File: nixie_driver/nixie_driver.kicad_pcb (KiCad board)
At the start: 2 copper layers, 39 parts, among them J1 USB_B_Micro, J14 Anode, J15 Number IO, J16 Number IO, J17 Anode, J18 Anode, J19 Number IO, J2 GPIO, J20 Number IO, J21 Anode, J22 Anode, J23 Number IO, J24 Number IO, J25 Anode, J3 HV_TEST, J4 Screw_Terminal_01x02, J5 Number IO, J6 Anode, J7 Number IO, J8 Anode, U1 SN74141N, U2 SN74141N, U3 SN74141N, U4 SN74141N

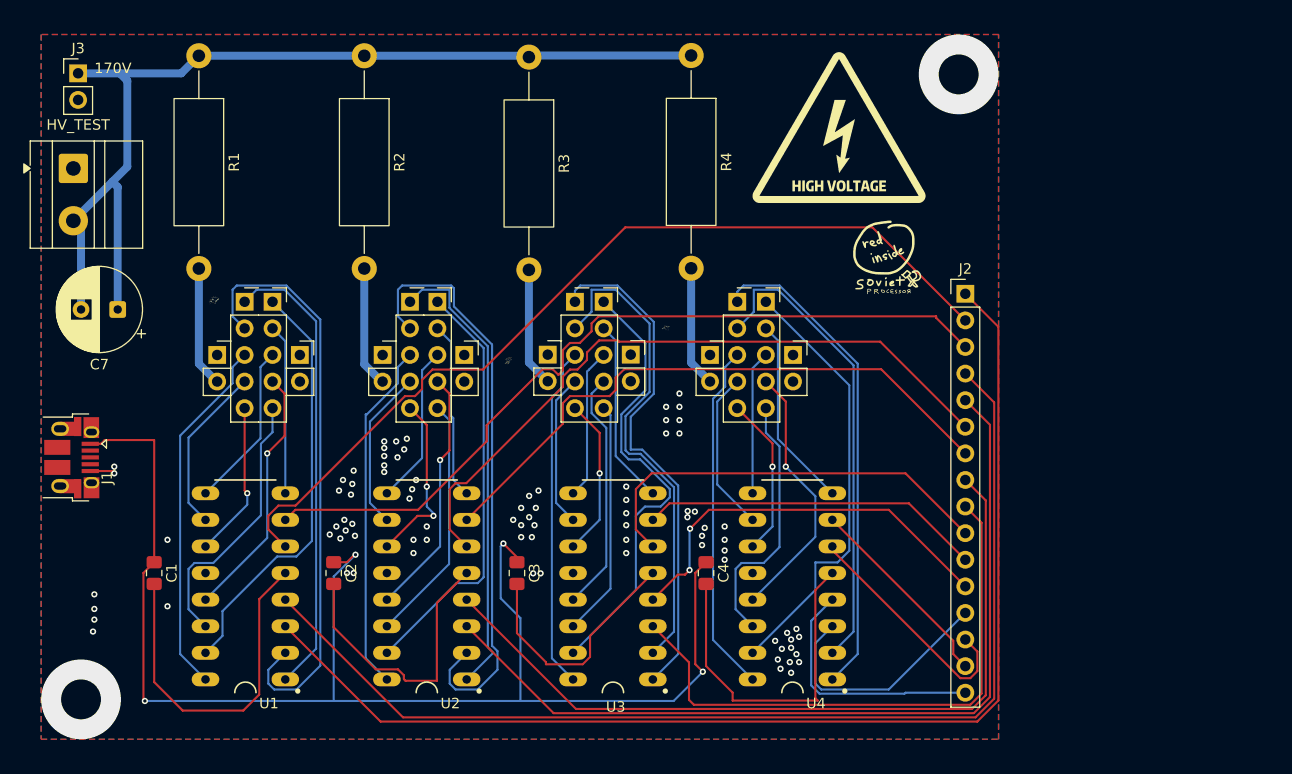
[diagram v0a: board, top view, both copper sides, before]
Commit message: updated pcb
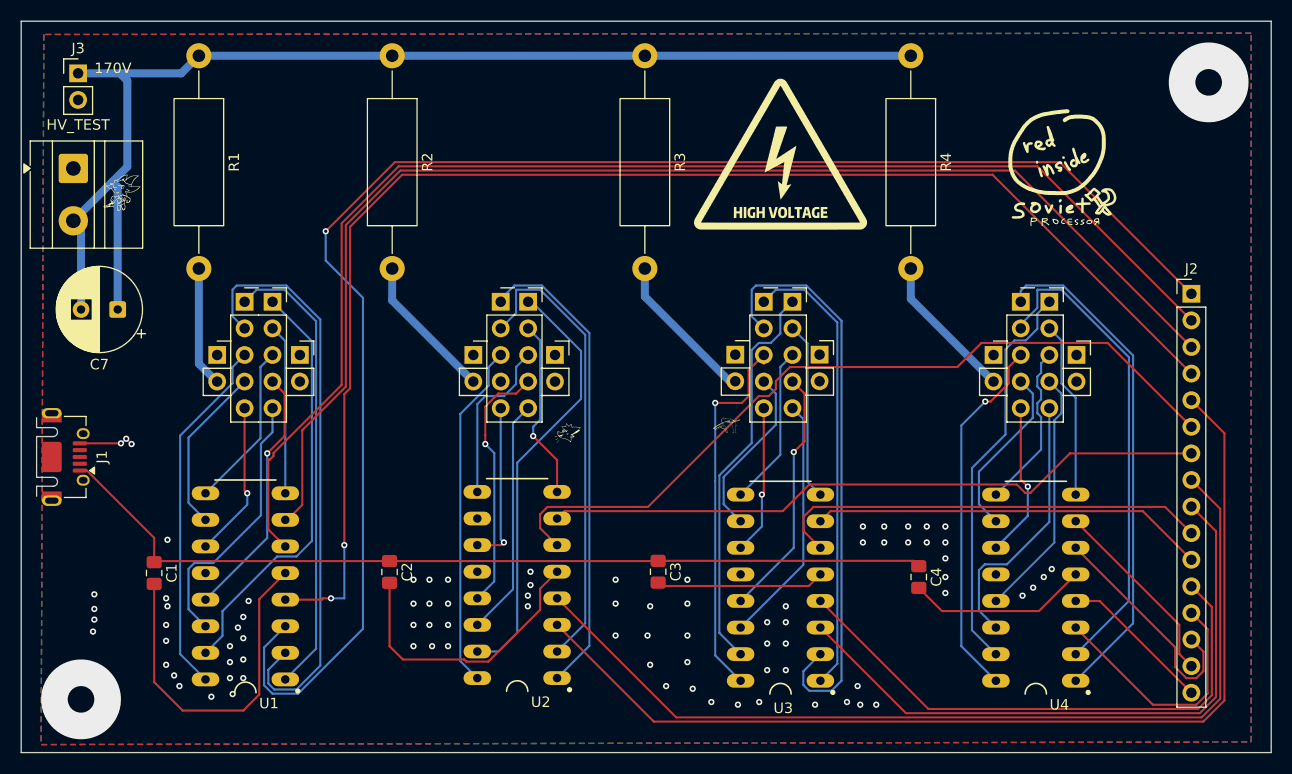
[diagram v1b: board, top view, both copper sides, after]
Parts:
- removed the G*** at (170.2, 73.7)
- removed the G*** at (191.1, 67.3)
- removed the G*** at (155.1, 76.8)
- removed the G*** at (127.0, 71.1)
- added G***: LOGO, logos:soviet_approved_big, F.Cu at (207.8, 58.9)
- added G***: LOGO, logos:bigger_shork_but_tiny, F.Cu at (160.8, 83.8)
- added G***: LOGO, logos:bigger_guy_but_small, F.Cu at (176.0, 82.8)
- added G***: LOGO, logos:thistlebig, F.Cu at (118.1, 60.7)
- J1: footprint Connector_USB:USB_Micro-B_Amphenol_10103594-0001LF_Horizontal -> Connector_USB:USB_Micro-AB_Molex_47590-0001
- moved G*** 31.5 mm to (168.5, 80.3)
- moved J22 27.1 mm to (201.4, 76.3)
- moved J23 27.1 mm to (204.0, 71.2)
- moved J24 27.1 mm to (206.8, 71.2)
- moved J25 27.1 mm to (209.4, 76.3)
- moved U4 23.2 mm to (205.5, 98.6)
- moved J2 21.6 mm to (220.3, 70.5)
- moved R4 21.0 mm to (193.5, 47.8)
- moved C4 20.3 mm to (194.3, 97.5)
- moved J19 18.0 mm to (179.5, 71.2)
- moved J20 18.0 mm to (182.2, 71.2)
- moved J21 18.0 mm to (184.8, 76.3)
- moved J18 17.9 mm to (176.8, 76.3)
- moved U3 16.0 mm to (181.1, 98.6)
- moved C3 13.5 mm to (169.4, 97.0)
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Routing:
- net /5V: track 132.7 -> 85.4 mm, vias 4 -> 0
- net /U1_C: track 77.2 -> 120.6 mm
- net /U1_B: track 85.8 -> 124.0 mm
- net /U1_A: track 112.9 -> 148.9 mm, vias 0 -> 1
- net /U1_D: track 105.3 -> 131.7 mm, vias 0 -> 2
- net 170V: track 101.6 -> 122.9 mm
- net Net-(U4-VCC): track 33.3 -> 17.4 mm
- net /U2_7: track 15.5 -> 0.00 mm
- net /U2_D: track 75.8 -> 90.8 mm
- net /U2_A: track 83.4 -> 98.4 mm
- net /U3_D: track 38.7 -> 53.4 mm, vias 2 -> 0
- net /U2_9: track 57.1 -> 44.0 mm
- net /U2_B: track 65.7 -> 76.4 mm
- net /U3_9: track 47.0 -> 56.6 mm
- net /U4_D: track 24.1 -> 14.7 mm
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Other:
- board outline added: 119.4 x 69.8 mm
